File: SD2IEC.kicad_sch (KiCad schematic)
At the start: 34 parts, among them J1 AVR-ISP-6, J2 5VDC IN, J3 SD_Card, J4 IEC (DIN6), J5 IEC (DIN6), J6 SERIAL, J7 I2C, J8 IEC_ALT1, J9 IEC_ALT2, SW1 IEC_SEL, SW2 PREV, SW3 NEXT, SW4 RESET, U1 ATmega1284P-20AU, U2 MIC5504-3.3YM5, Y1 8MHz

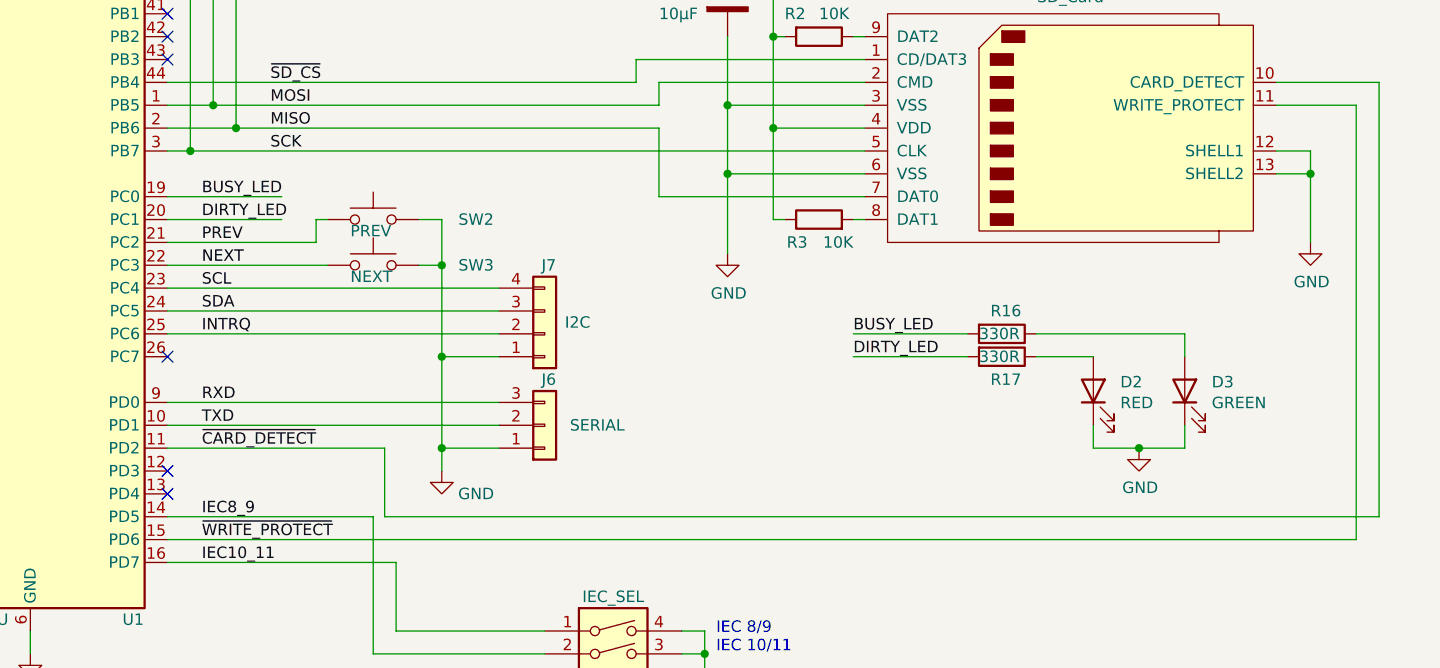
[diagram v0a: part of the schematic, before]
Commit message: Begin routing
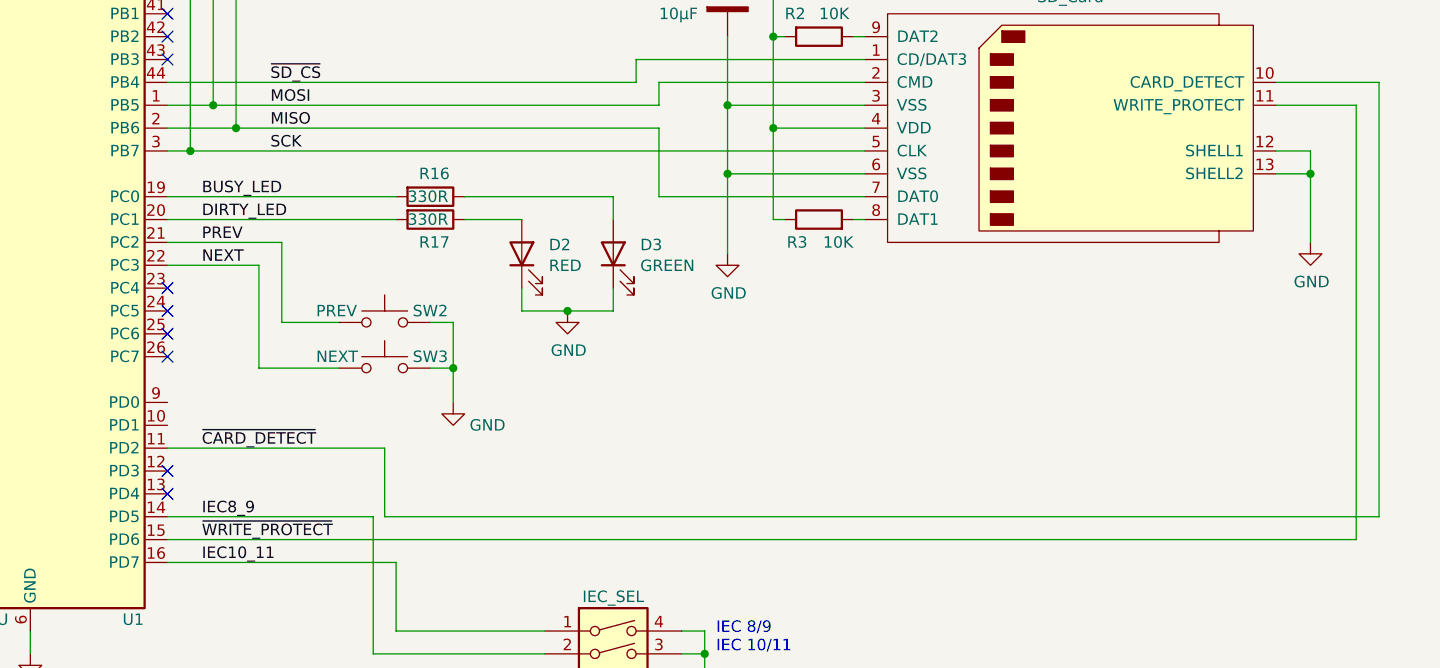
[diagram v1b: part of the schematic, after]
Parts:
- removed J6: SERIAL, Connector_PinHeader_2.54mm:PinHeader_1x03_P2.54mm_Vertical, symbol Connector_Generic:Conn_01x03
- removed J7: I2C, Connector_PinHeader_2.54mm:PinHeader_1x04_P2.54mm_Vertical, symbol Connector_Generic:Conn_01x04
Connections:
- net INTRQ: no longer names the net of U1.25 (PC6)
- net RXD: no longer names the net of U1.9 (PD0)
- net SCL: no longer names the net of U1.23 (PC4)
- net SDA: no longer names the net of U1.24 (PC5)
- net TXD: no longer names the net of U1.10 (PD1)
- no-connect marks 13 -> 16
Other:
- moved on the sheet: D2, D3, R16, R17, SW2, SW3
